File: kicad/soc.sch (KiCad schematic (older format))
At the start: 10 parts, among them J1 JACK_TRS_3PINS, J2 PS/2 Keyboard, J3 PS/2 Mouse, P1 LED MATRIX, P10 CODEC right, P11 CODEC inputs, P2 ALTERA_DE1_GPIO, P9 CODEC left, U2 DS3234

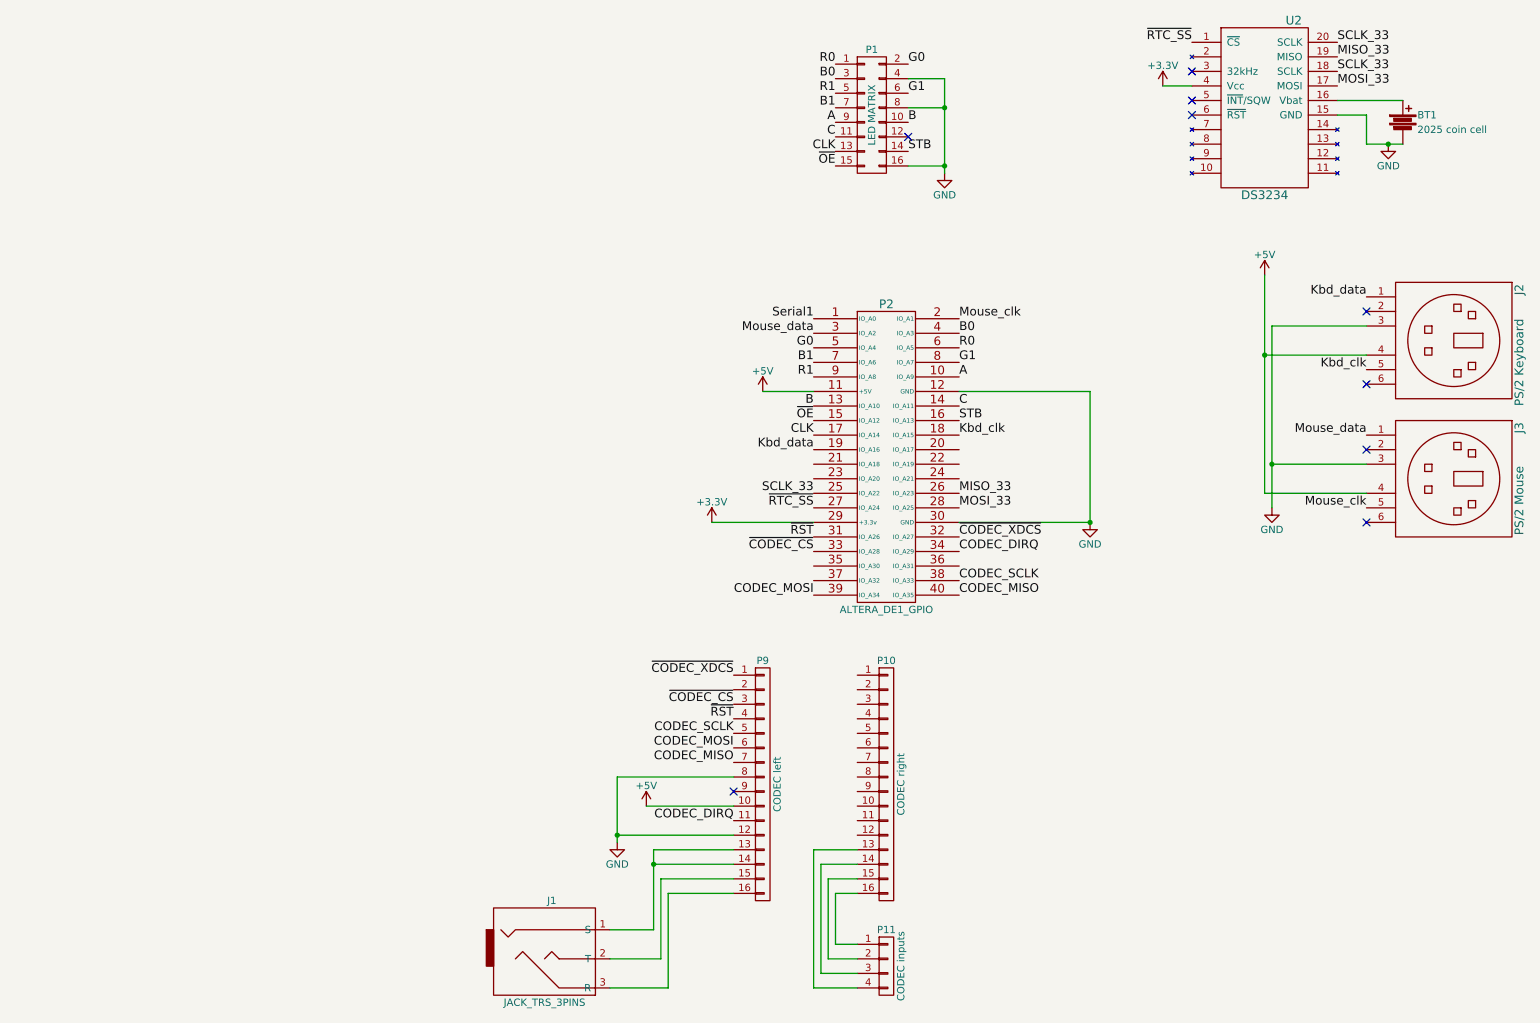
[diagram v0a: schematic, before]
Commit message: close to final
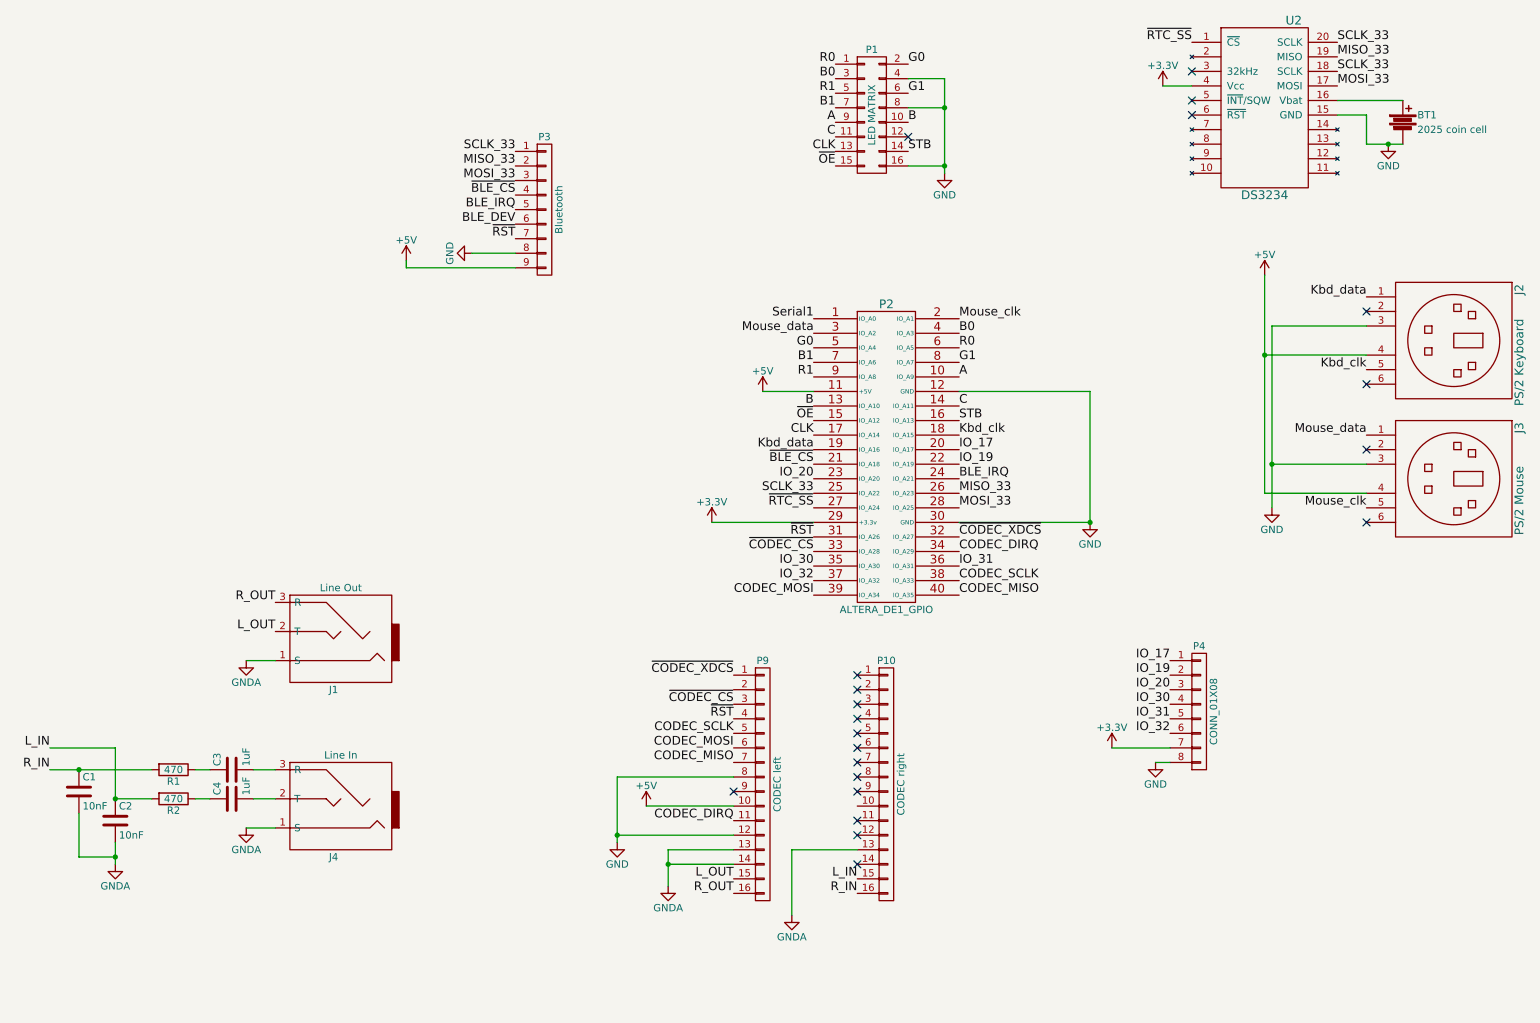
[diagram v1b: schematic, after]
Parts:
- removed P11: CODEC inputs, Pin_Headers:Pin_Header_Straight_1x04, symbol CONN_01X04
- added C1, C2: 10nF, Capacitors_SMD:C_0805_HandSoldering, symbol C
- added C3, C4: 1uF, Capacitors_SMD:C_0805_HandSoldering, symbol C
- added J4: Line In, mstock-pretty:SJI-3513N, symbol JACK_TRS_3PINS
- added P3: Bluetooth, Socket_Strips:Socket_Strip_Straight_1x09, symbol CONN_01X09
- added P4: CONN_01X08, Pin_Headers:Pin_Header_Straight_2x04, symbol CONN_01X08
- added R1, R2: 470, Resistors_SMD:R_0805_HandSoldering, symbol R
- J1: value JACK_TRS_3PINS -> Line Out
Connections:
- net +3V3: now also P4.7 (P7)
- net +5V: now also P3.9 (P9)
- net GND: now also P3.8 (P8), P4.8 (P8)
- net MISO_33: now also P3.2 (P2)
- net MOSI_33: now also P3.3 (P3)
- net SCLK_33: now also P3.1 (P1)
- net ~RST: now also P3.7 (P7)
- net IO_17: now reaches P2.20 (IO_A17)
- net IO_17: now also P4.1 (P1)
- net ~BLE_CS: now reaches P2.21 (IO_A18)
- net ~BLE_CS: now also P3.4 (P4)
- net IO_19: now reaches P2.22 (IO_A19)
- net IO_19: now also P4.2 (P2)
- net IO_20: now reaches P2.23 (IO_A20)
- net IO_20: now also P4.3 (P3)
- net BLE_IRQ: now reaches P2.24 (IO_A21)
- net BLE_IRQ: now also P3.5 (P5)
- net IO_30: now reaches P2.35 (IO_A30)
- net IO_30: now also P4.4 (P4)
- net IO_31: now reaches P2.36 (IO_A31)
- net IO_31: now also P4.5 (P5)
- net IO_32: now reaches P2.37 (IO_A32)
- net IO_32: now also P4.6 (P6)
- net GNDA: now reaches J1.1 (S), P9.13 (P13), P9.14 (P14)
- net GNDA: now also P10.13 (P13), C1.2, C2.2, J4.1 (S)
- net L_OUT: now reaches J1.2 (T), P9.15 (P15)
- net R_OUT: now reaches J1.3 (R), P9.16 (P16)
- net L_IN: now reaches P10.15 (P15)
- net L_IN: now also C2.1, R2.2
- net R_IN: now reaches P10.16 (P16)
- net R_IN: now also C1.1, R1.2
- new net: C4.2, J4.2 (T)
- new net: C3.2, J4.3 (R)
- new net: C3.1, R1.1
- new net: C4.1, R2.1
- new net BLE_DEV: P3.6 (P6)
- no-connect marks 9 -> 21
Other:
- moved on the sheet: J1

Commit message: Revert "close to final"
This reverts commit c876cf625f705db1e319b0381db18ed40929d998.
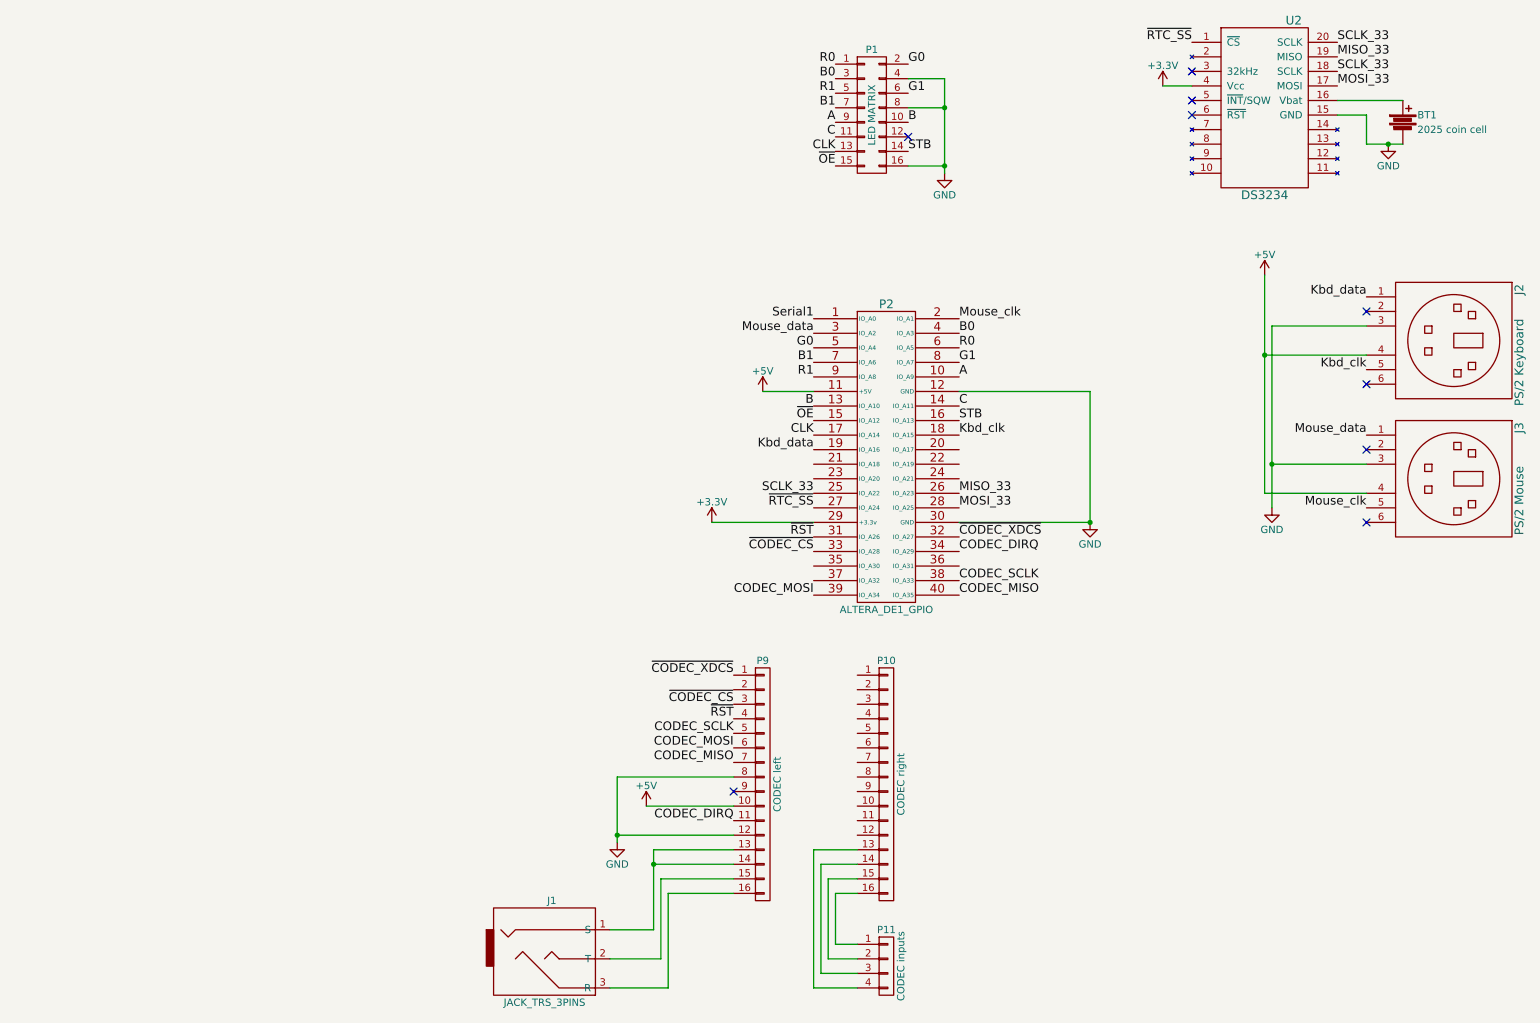
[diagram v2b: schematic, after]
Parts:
- removed C1, C2: 10nF, Capacitors_SMD:C_0805_HandSoldering, symbol C
- removed C3, C4: 1uF, Capacitors_SMD:C_0805_HandSoldering, symbol C
- removed J4: Line In, mstock-pretty:SJI-3513N, symbol JACK_TRS_3PINS
- removed P3: Bluetooth, Socket_Strips:Socket_Strip_Straight_1x09, symbol CONN_01X09
- removed P4: CONN_01X08, Pin_Headers:Pin_Header_Straight_2x04, symbol CONN_01X08
- removed R1, R2: 470, Resistors_SMD:R_0805_HandSoldering, symbol R
- added P11: CODEC inputs, Pin_Headers:Pin_Header_Straight_1x04, symbol CONN_01X04
- J1: value Line Out -> JACK_TRS_3PINS
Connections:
- net at P10.14 (P14): now also P11.3 (P3)
- net BLE_IRQ: no longer names the net of P2.24 (IO_A21)
- net GNDA: no longer names the net of J1.1 (S), P9.13 (P13), P9.14 (P14)
- net GNDA: no longer P10.13 (P13)
- net IO_17: no longer names the net of P2.20 (IO_A17)
- net IO_19: no longer names the net of P2.22 (IO_A19)
- net IO_20: no longer names the net of P2.23 (IO_A20)
- net IO_30: no longer names the net of P2.35 (IO_A30)
- net IO_31: no longer names the net of P2.36 (IO_A31)
- net IO_32: no longer names the net of P2.37 (IO_A32)
- net L_IN: no longer names the net of P10.15 (P15)
- net L_IN: now also P11.2 (P2)
- net L_OUT: no longer names the net of J1.2 (T), P9.15 (P15)
- net R_IN: no longer names the net of P10.16 (P16)
- net R_IN: now also P11.1 (P1)
- net R_OUT: no longer names the net of J1.3 (R), P9.16 (P16)
- net ~BLE_CS: no longer names the net of P2.21 (IO_A18)
- new net: P10.13 (P13), P11.4 (P4)
- no-connect marks 21 -> 9
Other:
- moved on the sheet: J1
